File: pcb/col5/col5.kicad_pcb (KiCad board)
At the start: 2 copper layers, 100.8 x 17.6 mm, 15 parts

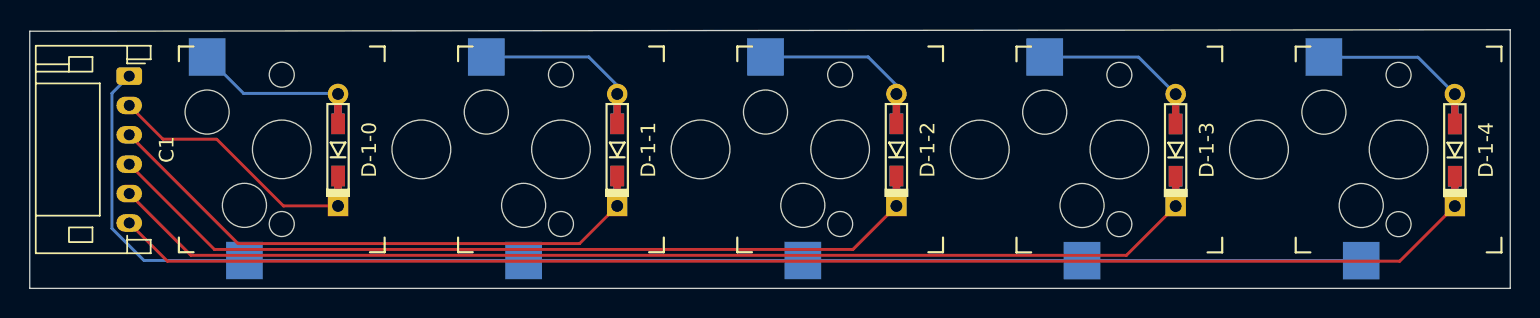
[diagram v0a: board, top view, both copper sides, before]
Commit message: adjusted  col unit pcb
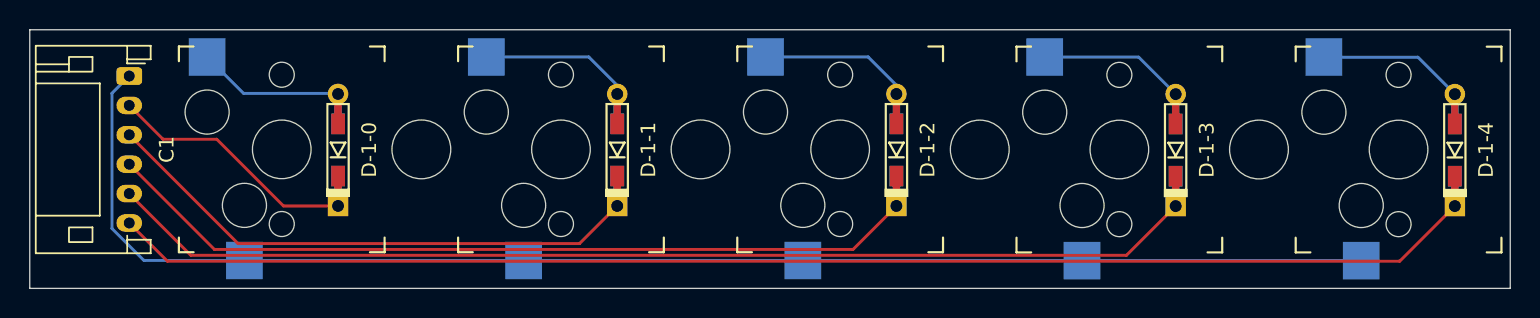
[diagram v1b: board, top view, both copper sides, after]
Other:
- outline, holes or cut-outs redrawn
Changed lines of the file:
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@@
 	)
 	(gr_line
-		(start 34.4 41.1)
+		(start 34.4 41)
 		(end 34.4 58.599958)
 		(stroke
@@
 	(gr_line
 		(start 135.15 41)
-		(end 34.4 41.1)
+		(end 34.4 41)
 		(stroke
 			(width 0.05)
@@
 	(gr_line
 		(start 135.15 58.6)
-		(end 34.4 58.599945)
+		(end 34.4 58.6)
 		(stroke
 			(width 0.05)
